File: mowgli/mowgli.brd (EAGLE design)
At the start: 72.4 x 23.6 mm, 19 parts, among them IC1 ATMEGA, IC2 MCP1702-33, X1 16 MHz, X2 uFL, X3 JSTPH

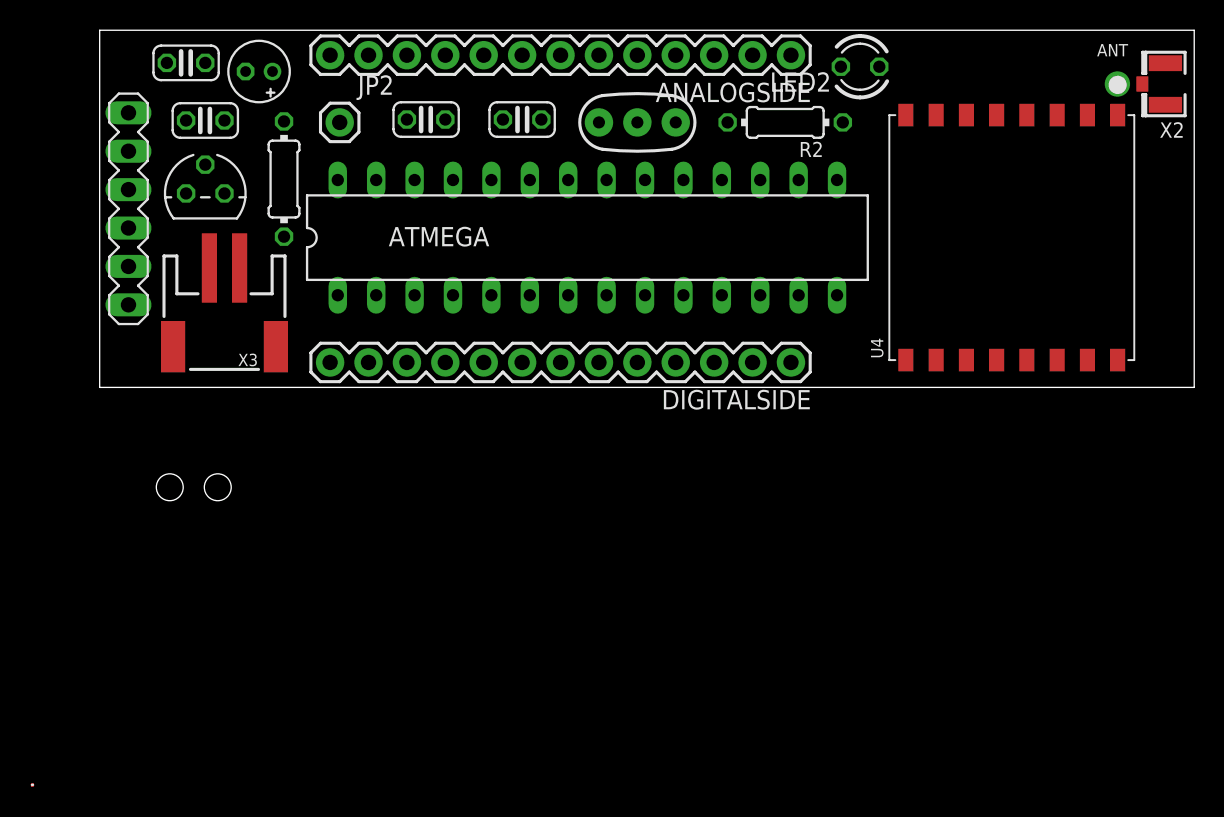
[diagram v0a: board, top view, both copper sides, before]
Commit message: update
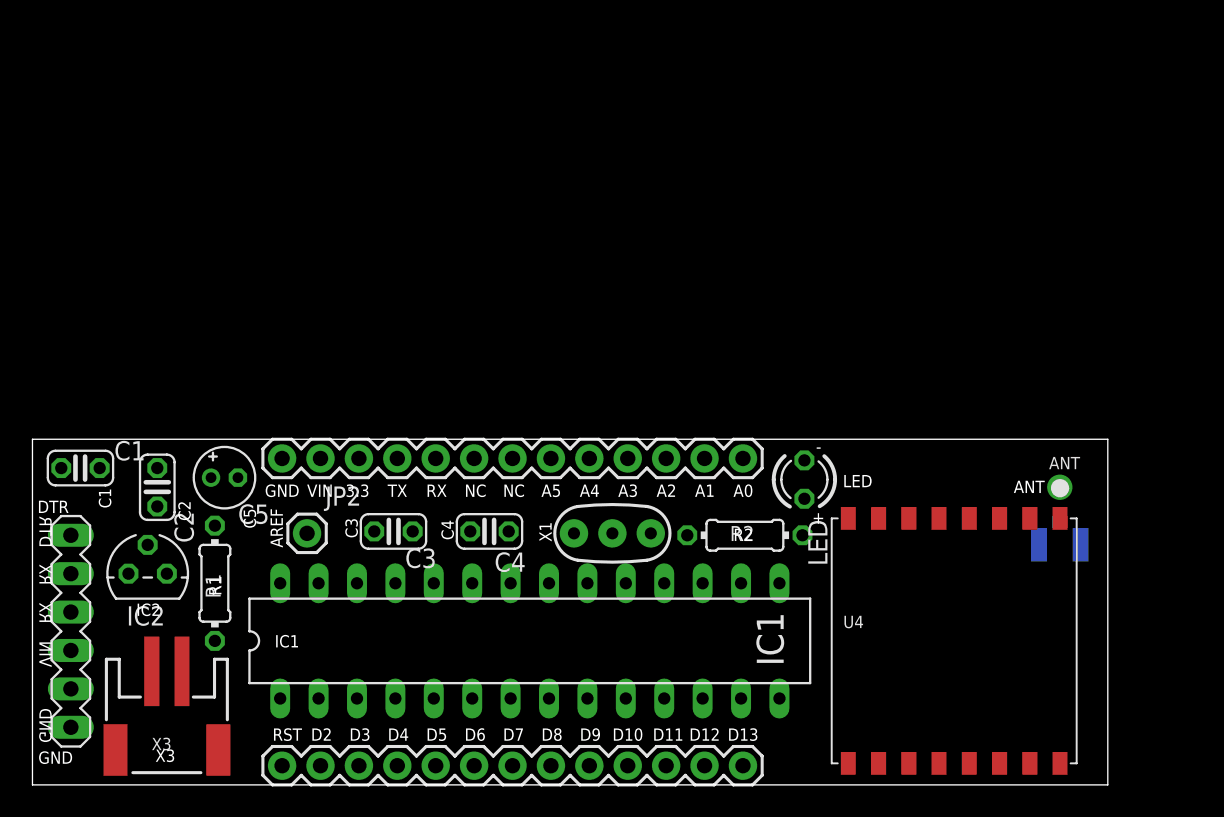
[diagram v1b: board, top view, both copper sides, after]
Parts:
- removed LED2: (no value), led:LED3MM
- added LED: (no value), led:LED3MM
- moved X2 31.3 mm to (67.9, 15.9), flipped to the bottom, turned to 90 degrees
- moved FTDI 28.2 mm to (2.54, 3.81)
- moved C1 27.7 mm to (3.17, 21.0)
- moved R2 27.4 mm to (47.1, 16.5)
- moved C3 27.3 mm to (23.9, 16.8), turned to 0 degrees
- moved C4 27.3 mm to (30.2, 16.8), turned to 180 degrees
- moved JP2 27.3 mm to (18.2, 16.6)
- moved X1 27.2 mm to (38.4, 16.6)
- moved R1 27.1 mm to (12.1, 13.3), turned to 270 degrees
- moved C5 27.0 mm to (12.7, 20.3), turned to 0 degrees
- moved IC1 26.9 mm to (32.9, 9.53)
- moved U4 26.9 mm to (61.0, 9.53)
- moved X3 26.9 mm to (8.89, 3.81)
- moved ANT 26.9 mm to (67.9, 19.7)
- moved DIGITALSIDE 26.9 mm to (47.0, 1.27)
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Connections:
- net GND: now also LED.K; no longer LED2.K
- net N$2: now also LED.A; no longer LED2.A
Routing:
- net N$14: track 1.09 -> 0.00 mm
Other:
- board size 72.4 x 23.6 mm -> 71.1 x 22.9 mm
- board text added: "+"
- board text added: "-"
- board text added: "3.3"
- board text added: "A0"
- board text added: "A1"
- board text added: "A2"
- board text added: "A3"
- board text added: "A4"
- board text added: "A5"
- board text added: "ANT"
- board text added: "AREF"
- board text added: "C1"
- board text added: "C2"
- board text added: "C3"
- board text added: "C4"
- board text added: "C5"
- board text added: "D10"
- board text added: "D11"
- board text added: "D12"
- board text added: "D13"
- board text added: "D2"
- board text added: "D3"
- board text added: "D4"
- board text added: "D5"
- board text added: "D6"
- board text added: "D7"
- board text added: "D8"
- board text added: "D9"
- board text added: "GND"
- board text added: "IC1"
- board text added: "IC2"
- board text added: "LED"
- board text added: "NC"
- board text added: "R1"
- board text added: "R2"
- board text added: "RST"
- board text added: "RX"
- board text added: "TX"
- board text added: "VIN"
- board text added: "X1"
- board text added: "X3"
